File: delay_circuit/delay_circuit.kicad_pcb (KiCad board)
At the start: 2 copper layers, 89.5 x 133 mm, 26 parts, among them J1 IN 12V AC, J2 OUT 230V AC, J3 IN 230V AC, J4 From Trfo Output, J5 OUT 5V CC, J6 To Power Ampli Power IN, J7 From Ampli Output, J8 OUT 12V CC, J9 To Speakers, K1 SANYOU_SRD_Form_C, K2 SANYOU_SRD_Form_C, Q1 NPN, Q2 NPN, U1 LM7812_TO220

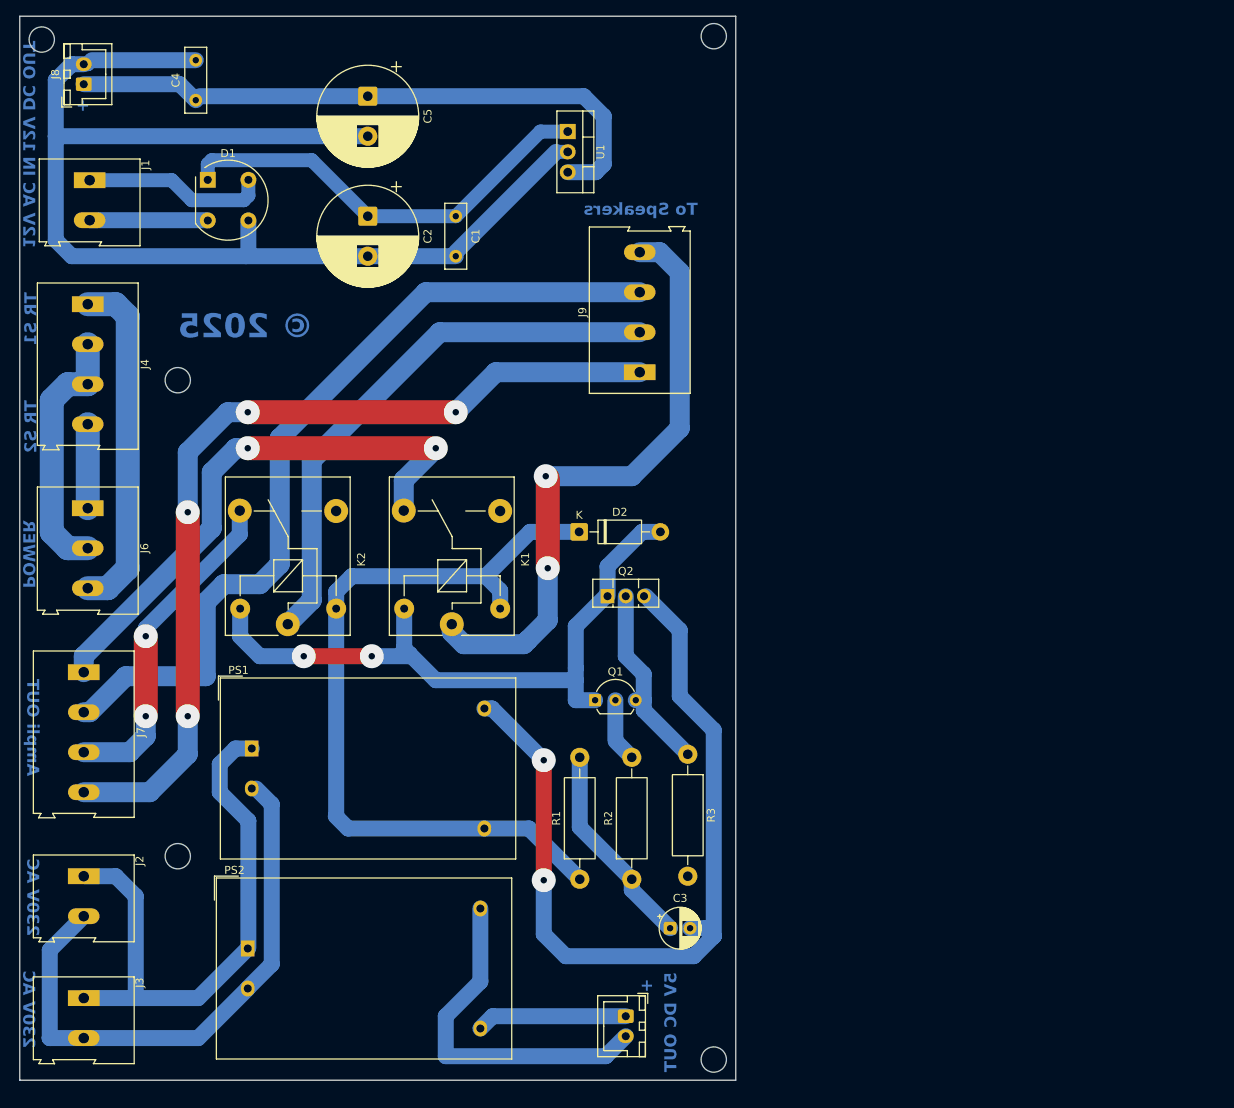
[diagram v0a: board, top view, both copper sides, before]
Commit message: Updated board
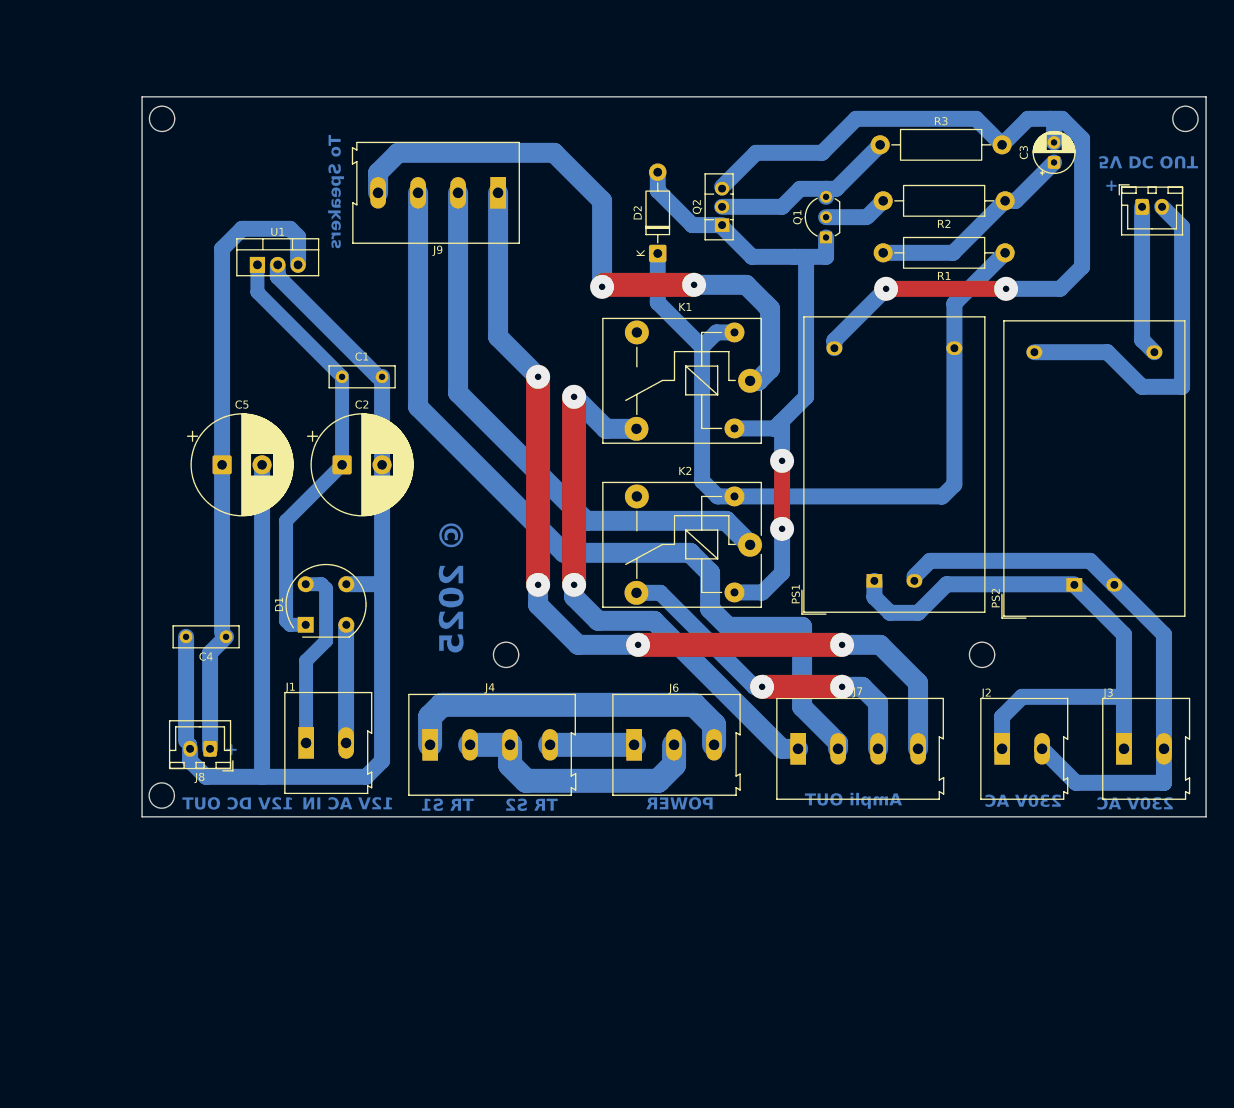
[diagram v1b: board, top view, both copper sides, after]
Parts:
- moved J3 133.7 mm to (157.3, 106.6), turned to 0 degrees
- moved J5 120.0 mm to (159.5, 38.8), turned to 0 degrees
- moved J2 115.9 mm to (142.0, 106.6), turned to 0 degrees
- moved PS2 112.9 mm to (151.1, 86.1), turned to 90 degrees
- moved C3 107.1 mm to (148.5, 33.3), turned to 90 degrees
- moved R2 96.8 mm to (142.4, 38.1), turned to 180 degrees
- moved R1 94.6 mm to (142.4, 44.6), turned to 180 degrees
- moved J7 89.8 mm to (116.5, 106.6), turned to 0 degrees
- moved J8 84.6 mm to (43.0, 106.6), turned to 180 degrees
- moved PS1 80.6 mm to (126.1, 85.6), turned to 90 degrees
- moved R3 79.9 mm to (126.8, 31.1), turned to 0 degrees
- moved J1 75.4 mm to (55.0, 105.8), turned to 0 degrees
- moved J6 74.4 mm to (96.0, 106.1), turned to 0 degrees
- moved J4 69.7 mm to (70.5, 106.1), turned to 0 degrees
- moved C4 67.2 mm to (45.0, 92.6), turned to 180 degrees
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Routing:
- net 0: track 105.3 -> 107.4 mm
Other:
- board size 89.5 x 133 mm -> 133 x 90 mm
